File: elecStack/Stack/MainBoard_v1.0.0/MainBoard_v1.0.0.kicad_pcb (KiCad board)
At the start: 2 copper layers, 168 x 138.5 mm, 59 parts, among them J1 Conn_01x04_Socket, J10 Conn_01x02_Socket, J2 Conn_01x06_Pin, J3 Conn_01x06_Pin, J4 Conn_01x02_Socket, J5 Conn_01x02_Socket, J6 Conn_01x07_Pin, J8 Conn_01x02_Socket, J9 Conn_01x02_Socket, Q1 NMOS, Q2 NMOS, Q3 NMOS, Q4 NMOS, Q5 NMOS, Q6 NMOS, Q7 NMOS, Q8 PMOS, SW1 SW_Push, SW2 SW_Wuerth_450301014042, U1 RASPBERRY_PI_PICO, U2 L293D, U3 TXS0108EPW, U4 L293D, U6 L293D

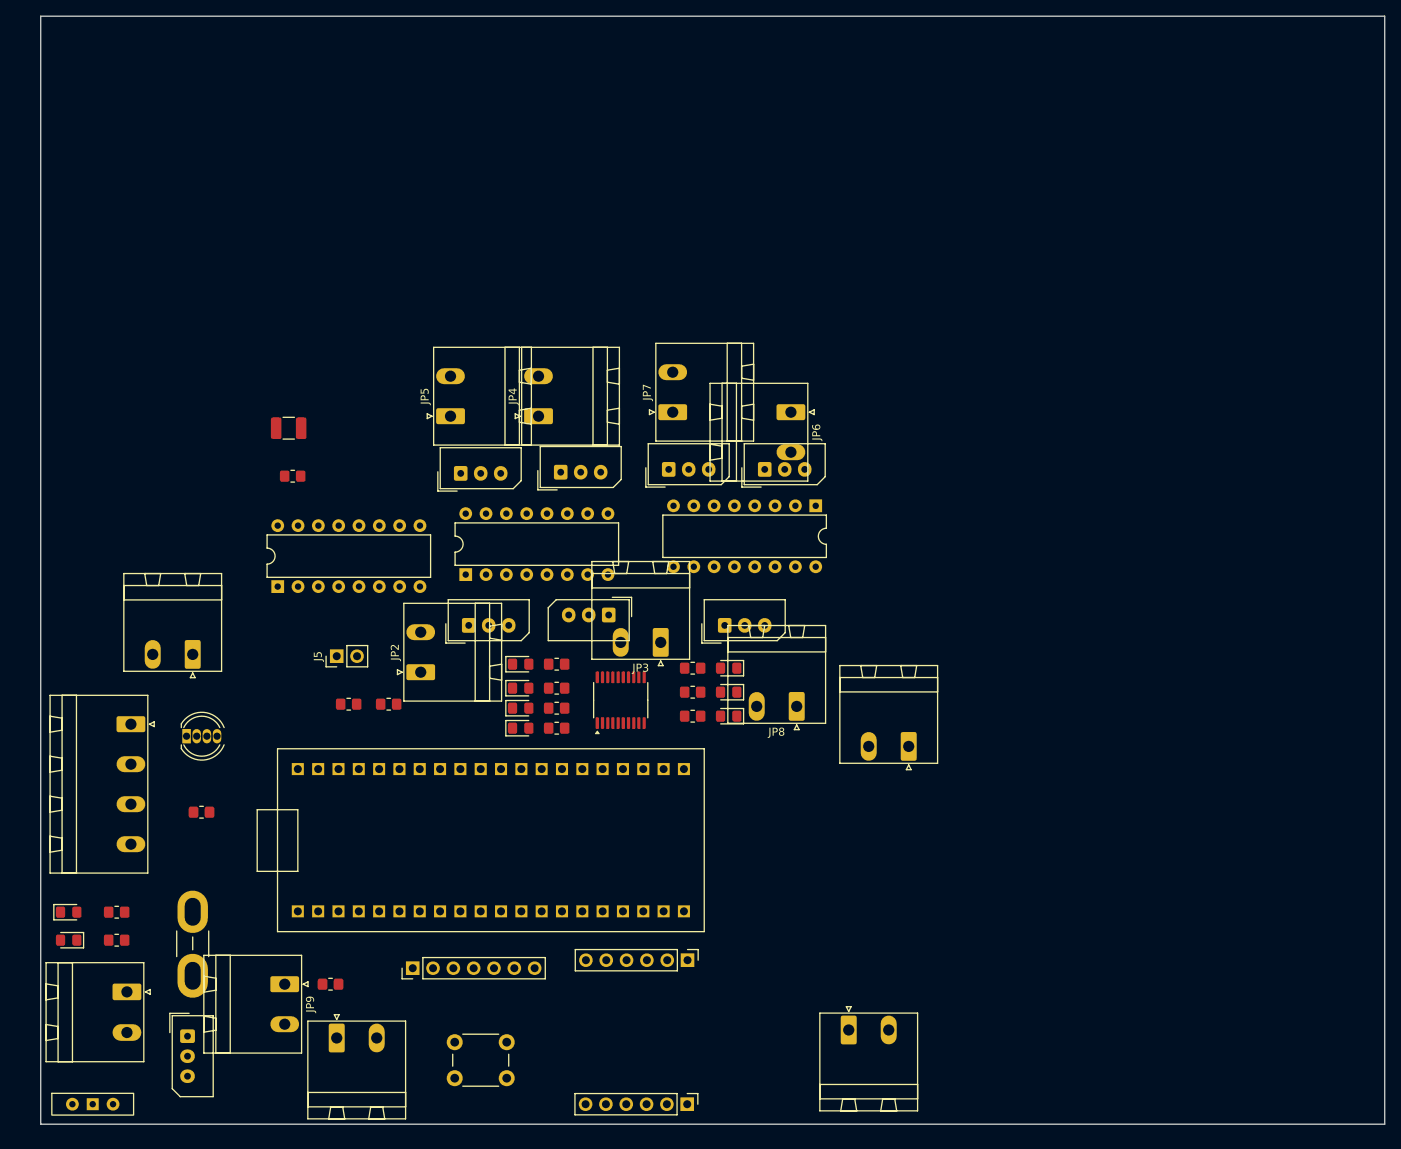
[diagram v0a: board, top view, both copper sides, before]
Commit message: Routing done
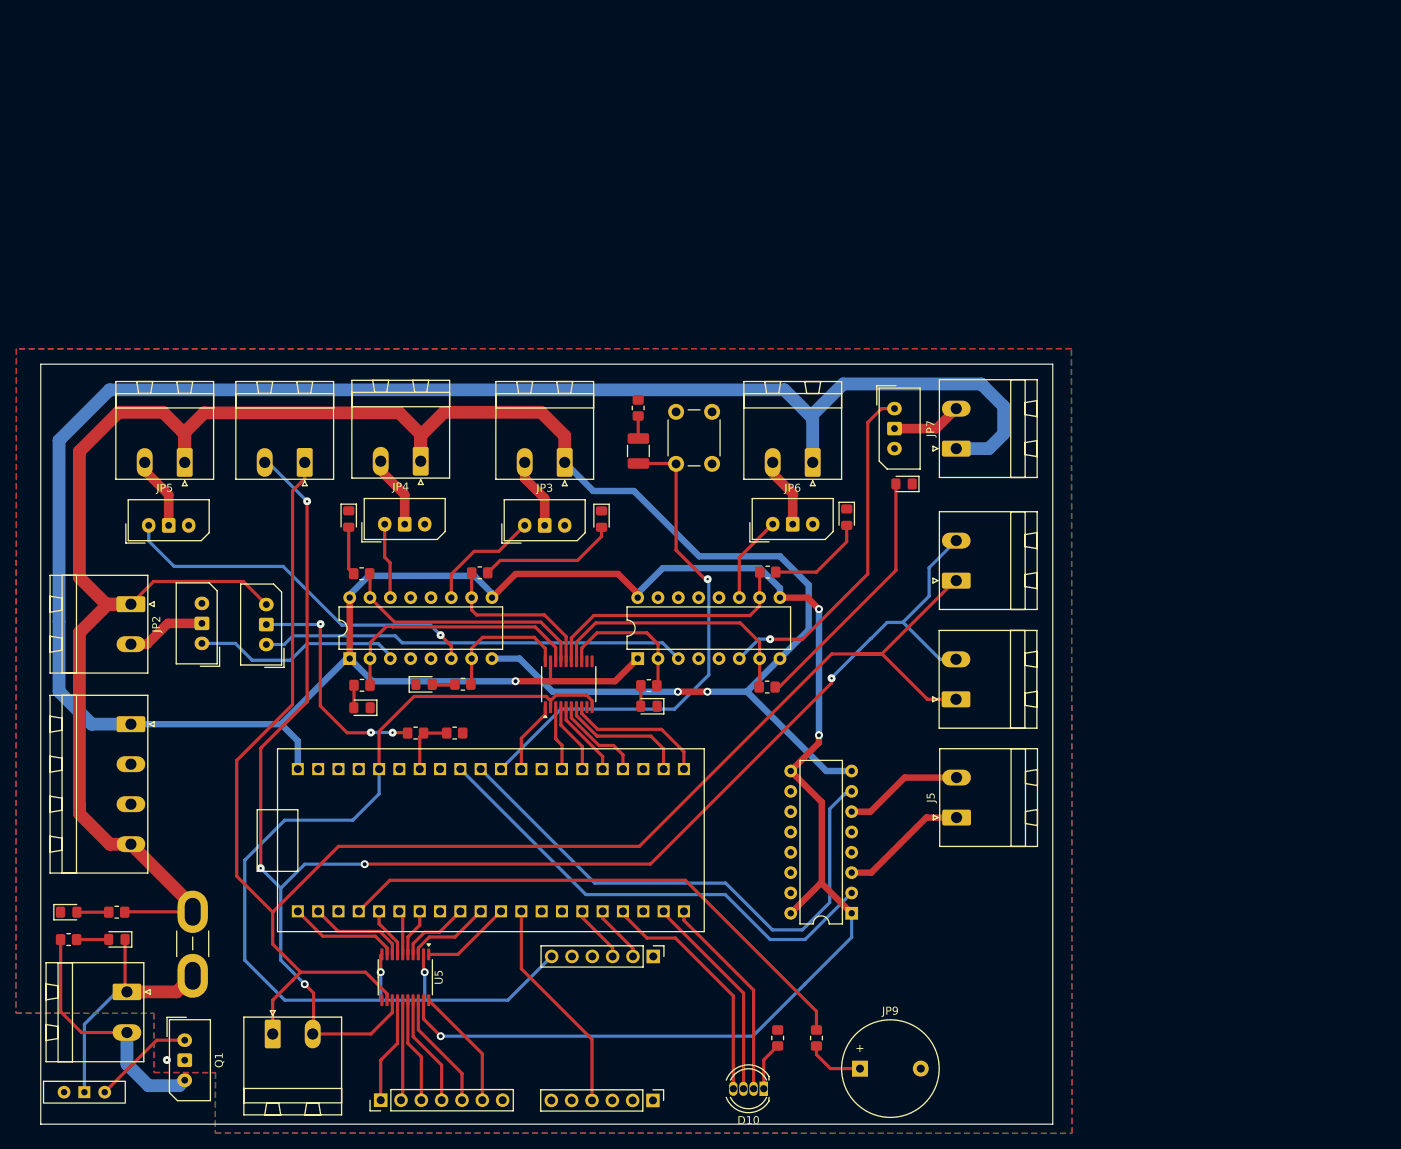
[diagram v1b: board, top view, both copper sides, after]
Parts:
- removed JP8: Jumper_2_Open, Connector_Phoenix_MSTB:PhoenixContact_MSTBA_2,5_2-G_1x02_P5.00mm_Horizontal
- added U5: TXS0108EPW, Package_SO:TSSOP-20_4.4x6.5mm_P0.65mm, F.Cu at (97.1, 143.6)
- D10: value APA-106-F5 -> ASMB-MTB0-0A3A2
- J5: footprint Connector_PinHeader_2.54mm:PinHeader_1x02_P2.54mm_Vertical -> Connector_Phoenix_MSTB:PhoenixContact_MSTBA_2,5_2-G_1x02_P5.00mm_Horizontal
- JP9: footprint Connector_Phoenix_MSTB:PhoenixContact_MSTBA_2,5_2-G_1x02_P5.00mm_Horizontal -> Buzzer_Beeper:Buzzer_12x9.5RM7.6
- Q1: footprint Connector_Molex:IRF540N -> Connector_Molex:Molex_SPOX_5267-03A_1x03_P2.50mm_Vertical
- moved D10 84.5 mm to (141.9, 157.6), turned to 180 degrees
- moved U6 82.6 mm to (152.9, 135.6), turned to 180 degrees
- moved J5 80.1 mm to (166.0, 123.7)
- moved SW1 77.4 mm to (130.9, 79.5), turned to 90 degrees
- moved R14 77.4 mm to (143.6, 151.2), turned to 90 degrees
- moved JP9 72.7 mm to (153.9, 155.1), turned to 0 degrees
- moved R3 61.1 mm to (148.5, 151.2), turned to -90 degrees
- moved J10 57.8 mm to (165.9, 94.0), turned to 90 degrees
- moved Q8 57.3 mm to (79.7, 102.0), turned to 90 degrees
- moved D5 52.2 mm to (90.0, 86.3), turned to -90 degrees
- moved D7 48.5 mm to (152.2, 86.1), turned to -90 degrees
- moved R13 44.0 mm to (126.2, 72.5), turned to -90 degrees
- moved R8 44.0 mm to (91.6, 93.2), turned to 180 degrees
- moved C1 43.8 mm to (126.2, 77.8), turned to -90 degrees
- moved Q5 39.5 mm to (65.0, 87.2)
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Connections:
- net DATA_IN renamed LED_PIN_1
- D10 pad 1: DATA_OUT -> Net-(D10-A)
- D10 pad 2: Net-(D10-GND) -> LED_PIN_3
- D10 pad 3: 3V3 -> LED_PIN_2
- J1 pad 1: PWR_IN -> 5V_buck
- J1 pad 2: GND_battery -> GND
- J1 pad 3: 5V_buck -> GND
- J1 pad 4: GND -> PWR_IN
- J10 pad 1: TXD_MD -> TXD_MD_5V
- J10 pad 2: RXD_MD -> RXD_MD_5V
- J3 pad 1: INT -> unconnected-(J3-Pin_1-Pad1)
- J4 pad 1: TXD_MD -> TXD_MD_5V
- J4 pad 2: RXD_MD -> RXD_MD_5V
- J6 pad 1: GP3 -> GP3_5V
- J6 pad 2: GP4 -> GP4_5V
- J6 pad 3: GP5 -> GP5_5V
- J6 pad 4: GP6 -> GP6_5V
- J6 pad 5: GP7 -> GP7_5V
- J6 pad 6: GP9 -> GP8_5V
- J6 pad 7: GP15 -> GND
- J8 pad 1: TXD_MD -> TXD_MD_5V
- J8 pad 2: RXD_MD -> RXD_MD_5V
- J9 pad 1: TXD_MD -> TXD_MD_5V
- J9 pad 2: RXD_MD -> RXD_MD_5V
- JP6 pad 1: 5V_Buck -> 5V_buck
- JP7 pad 1: 5V_Buck -> 5V_buck
- Q2 pad 2: G1 -> G2
- Q3 pad 2: G2 -> G4
- Q5 pad 2: G4 -> G1
- Q8 pad 3: Net-(JP8-B) -> PWR_IN
- R14 pad 1: GND -> Net-(D10-A)
- R14 pad 2: Net-(D10-GND) -> GND
- U1 pad GP10: INT -> unconnected-(U1-PadGP10)
- U1 pad GP14: DATA_OUT -> LED_PIN_2
- U1 pad GP15: GP15 -> LED_PIN_3
- U1 pad GP26_A0: TOGG_ACT_2 -> TOGG_ACT_1
- U1 pad GP27_A1: TOGG_ACT_1 -> TOGG_ACT_2
- U1 pad GP8: RST -> GP8
- U1 pad GP9: GP9 -> RST
- U2 pad 10: 5V_LVL_SHFT_3 -> 5V_LVL_SHFT_4
- U2 pad 11: G3 -> G4
- U2 pad 14: G4 -> G3
- U2 pad 15: 5V_LVL_SHFT_4 -> 5V_LVL_SHFT_3
- U2 pad 2: 5V_LVL_SHFT_1 -> 5V_LVL_SHFT_2
- U2 pad 3: G1 -> G2
- U2 pad 6: G2 -> G1
- U2 pad 7: 5V_LVL_SHFT_2 -> 5V_LVL_SHFT_1
- U3 pad 19: 5V_REF -> 5V_buck
- U4 pad 1: 3V3 -> 5V_buck
- U4 pad 10: 5V_LVL_SHFT_BATT -> 5V_LVL_SHFT_5
- U4 pad 11: G7 -> G5
- U4 pad 2: 5V_LVL_SHFT_5 -> 5V_LVL_SHFT_BATT
- U4 pad 3: G5 -> G7
- U4 pad 9: 3V3 -> 5V_buck
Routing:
- net 5V_buck: track 0.00 -> 450.5 mm, vias 0 -> 4
- net PWR_IN: track 0.00 -> 291.6 mm, vias 0 -> 2
- net TXD_MD_5V: track 0.00 -> 210.8 mm
- net RXD_MD_5V: track 0.00 -> 206.1 mm, vias 0 -> 5
- net 3V3: track 0.00 -> 125.6 mm, vias 0 -> 2
- net TOGG_ACT_1: track 0.00 -> 68.7 mm
- net BUZZ: track 0.00 -> 67.9 mm
- net RESET: track 0.00 -> 63.8 mm, vias 0 -> 1
- net TOGG_ACT_2: track 0.00 -> 60.1 mm
- net G7: track 0.00 -> 53.1 mm
- net G1: track 0.00 -> 46.8 mm, vias 0 -> 1
- net G6: track 0.00 -> 43.4 mm, vias 0 -> 1
- net 5V_LVL_SHFT_6: track 0.00 -> 32.9 mm
- net 5V_LVL_SHFT_5: track 0.00 -> 32.3 mm
- net 5V_LVL_SHFT_2: track 0.00 -> 32.2 mm
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- added copper zone on B.Cu, net GND
- added copper zone on F.Cu, net GND
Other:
- board size 168 x 138.5 mm -> 126.5 x 95 mm
